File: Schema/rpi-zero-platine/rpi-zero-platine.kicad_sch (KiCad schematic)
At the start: 4 parts, among them J1 GPIO, J2 Screw_Terminal_01x06, J3 Screw_Terminal_01x02, SW1 SW_DIP_x02

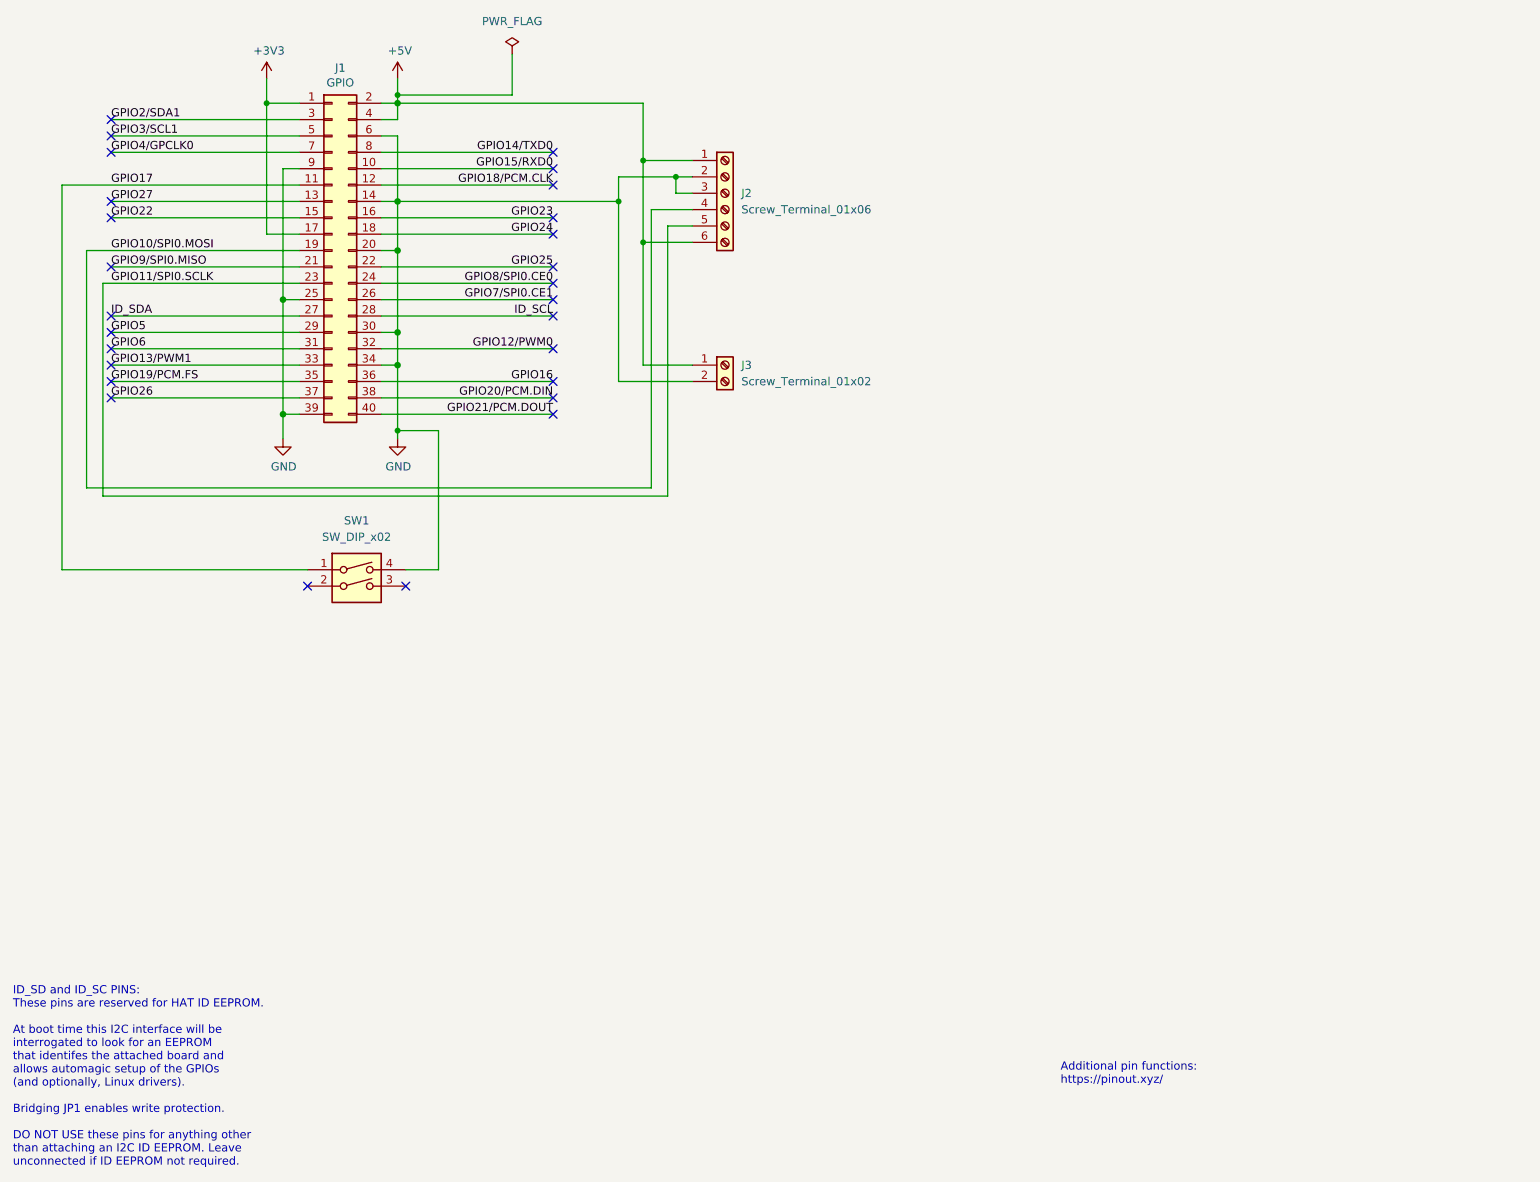
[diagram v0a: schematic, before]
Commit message: Überarbeite Platine
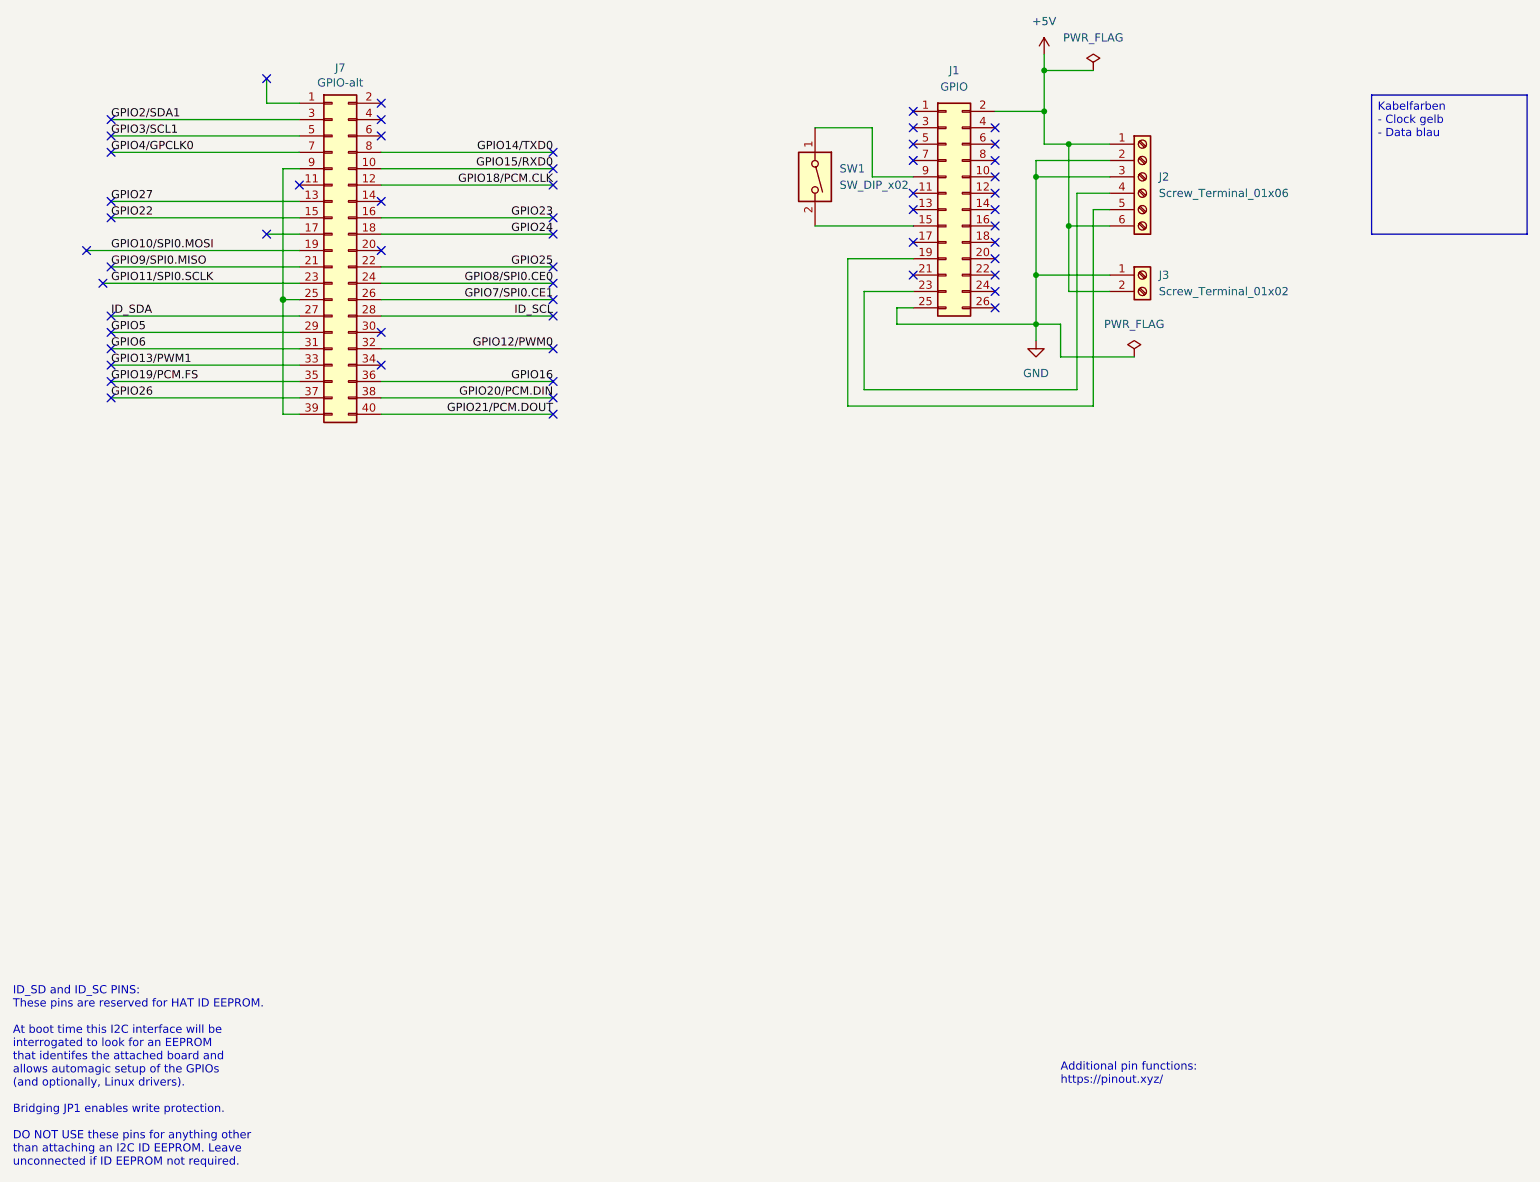
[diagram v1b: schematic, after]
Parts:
- added J1: GPIO, Connector_PinSocket_2.54mm:PinSocket_2x13_P2.54mm_Vertical, symbol Connector_Generic:Conn_02x13_Odd_Even
- J2: footprint TerminalBlock_Altech:Altech_AK100_1x06_P5.00mm -> TerminalBlock_Phoenix:TerminalBlock_Phoenix_MKDS-1,5-6-5.08_1x06_P5.08mm_Horizontal
- J3: footprint TerminalBlock:TerminalBlock_Altech_AK300-2_P5.00mm -> TerminalBlock_Phoenix:TerminalBlock_Phoenix_MKDS-1,5-2-5.08_1x02_P5.08mm_Horizontal
- J7: renamed from J1; value GPIO -> GPIO-alt
- SW1: footprint Button_Switch_THT:SW_DIP_SPSTx02_Piano_10.8x6.64mm_W7.62mm_P2.54mm -> Button_Switch_THT:SW_PUSH_6mm_H4.3mm; symbol Switch:SW_DIP_x02 -> Switch:SW_DIP_x01
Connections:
- net +5V: now also J3.2 (Pin_2), J1.2 (VCC); no longer J3.1 (Pin_1), J7.2 (Pin_2), J7.4 (Pin_4)
- net GND: now also J3.1 (Pin_1), J1.25 (GND); no longer J3.2 (Pin_2), J7.14 (Pin_14), J7.20 (Pin_20), J7.25 (Pin_25), J7.30 (Pin_30), J7.34 (Pin_34), J7.39 (Pin_39), J7.6 (Pin_6), J7.9 (Pin_9), SW1.4
- net GPIO10/SPI0.MOSI: no longer J2.4 (Pin_4)
- net GPIO11/SPI0.SCLK: no longer J2.5 (Pin_5)
- net at SW1.2: now also J1.15 (Pin_15)
- net +3V3: no longer names the net of J7.1 (Pin_1)
- net +3V3: no longer J7.17 (Pin_17)
- net GPIO17: no longer names the net of J7.11 (Pin_11)
- net GPIO17: no longer SW1.1
- new net: J7.25 (Pin_25), J7.39 (Pin_39), J7.9 (Pin_9)
- new net: J1.19 (SPI0.MOSI), J2.5 (Pin_5)
- new net: J1.23 (SPI0.SCLK), J2.4 (Pin_4)
- new net: J1.9 (Pin_9), SW1.1
- no-connect marks 27 -> 57
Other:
- moved on the sheet: J2, J3
